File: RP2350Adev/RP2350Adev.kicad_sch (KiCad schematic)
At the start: 43 parts, among them J1 USB4105-GF-A, J2 LEFT, J3 DEBUG, J4 RIGHT, U1 W25Q32JV, U2 RP2350A, U3 MCP1702T-3302E_CB, X1 IQXO-791

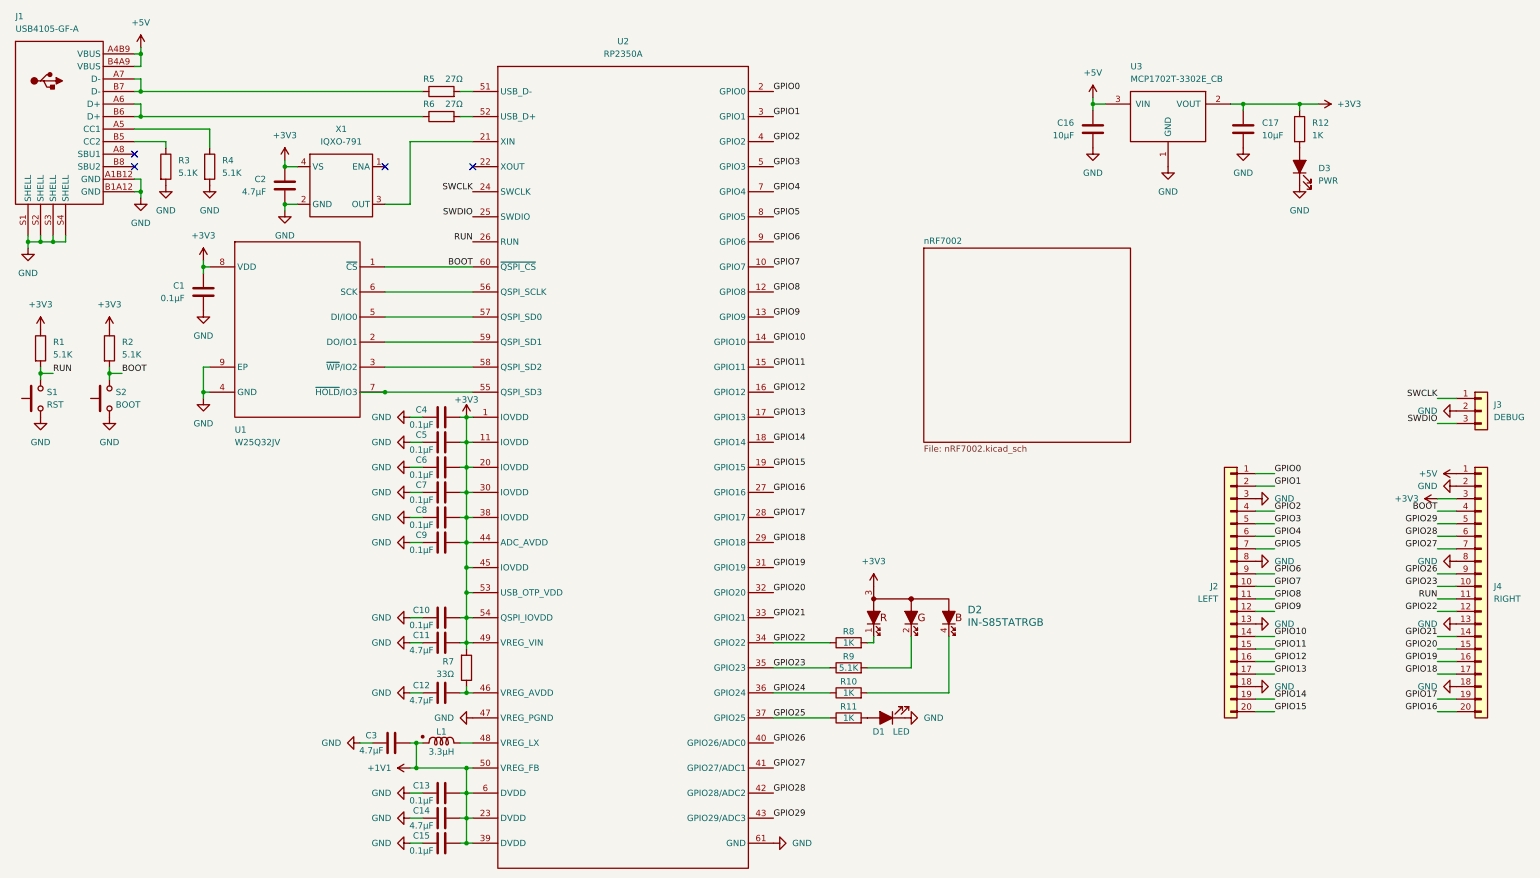
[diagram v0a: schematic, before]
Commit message: Muxful beginnings
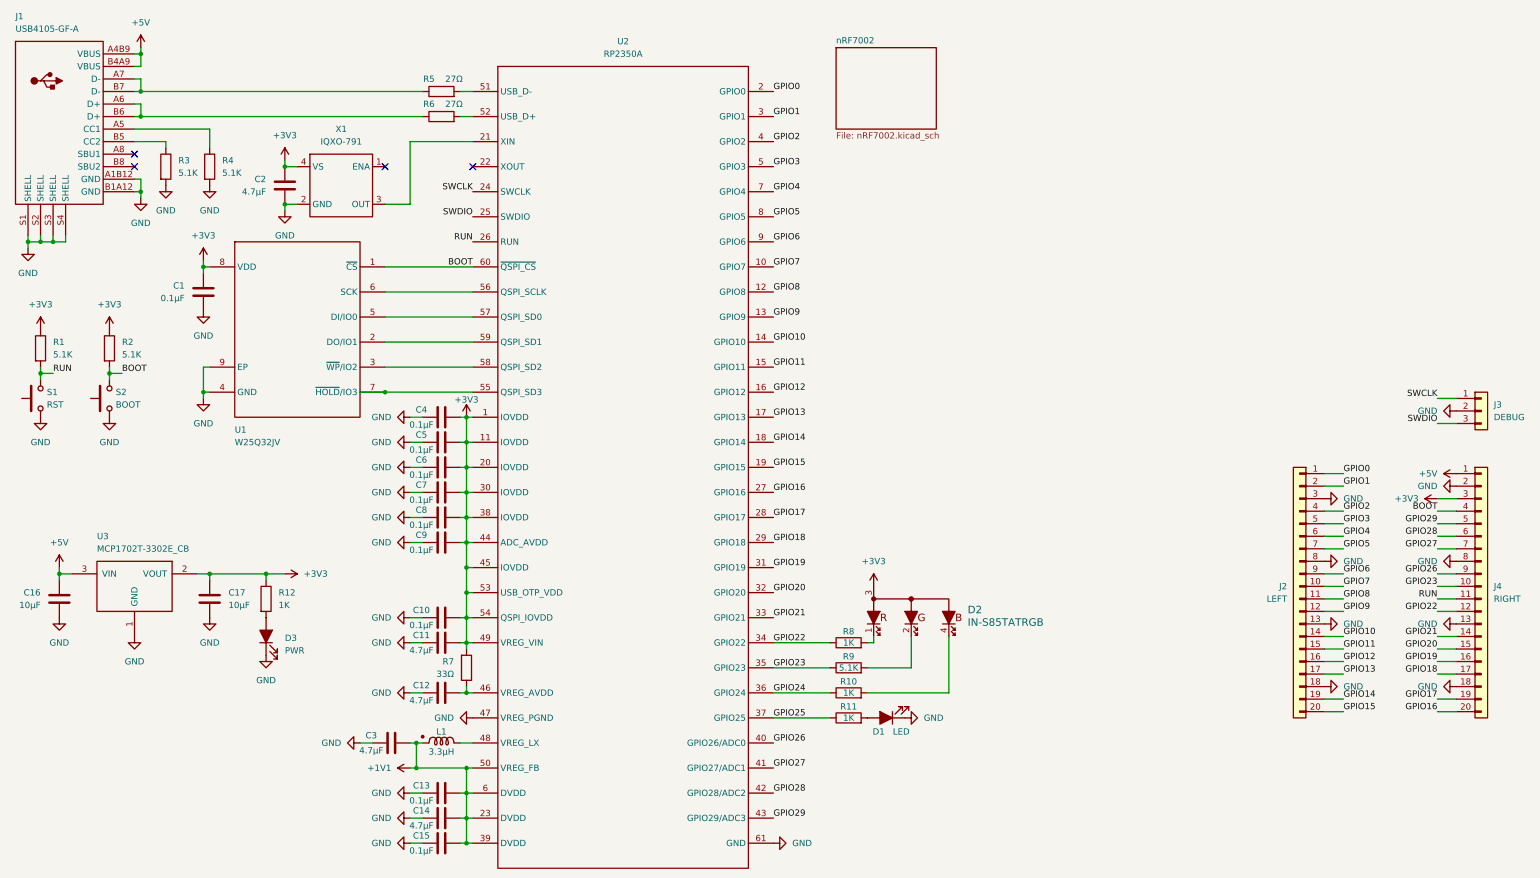
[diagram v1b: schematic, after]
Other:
- moved on the sheet: C16, C17, D3, J2, R12, U3
